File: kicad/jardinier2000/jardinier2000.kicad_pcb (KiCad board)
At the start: 2 copper layers, 54 parts, among them J1 5V, J10 I2C, J11 I2C, J12 Barrel_Jack_Switch, J2 VIN Reg, J3 5V, J4 5V, J5 5V, J6 5_30V, J7 I2C, J8 5V, J9 I2C, Q1 AO3400A, Q2 AO3400A, Q3 AO3400A, Q4 AO3400A, Q5 AO3400A, Q6 AO3400A, U1 ESP32_DevKit_V1_DOIT, U2 NCP1117-3.3_SOT223, U3 TPS62933P

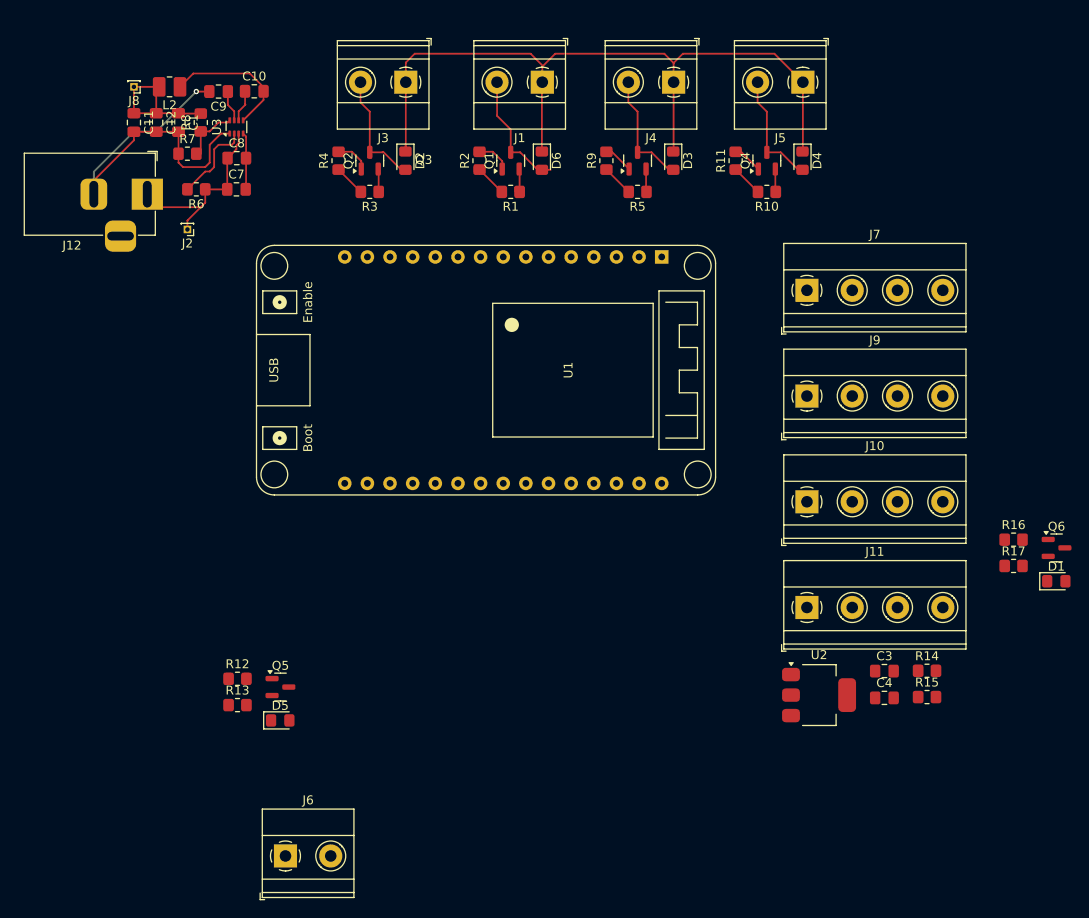
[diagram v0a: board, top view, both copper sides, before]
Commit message: Finished routing v1.0
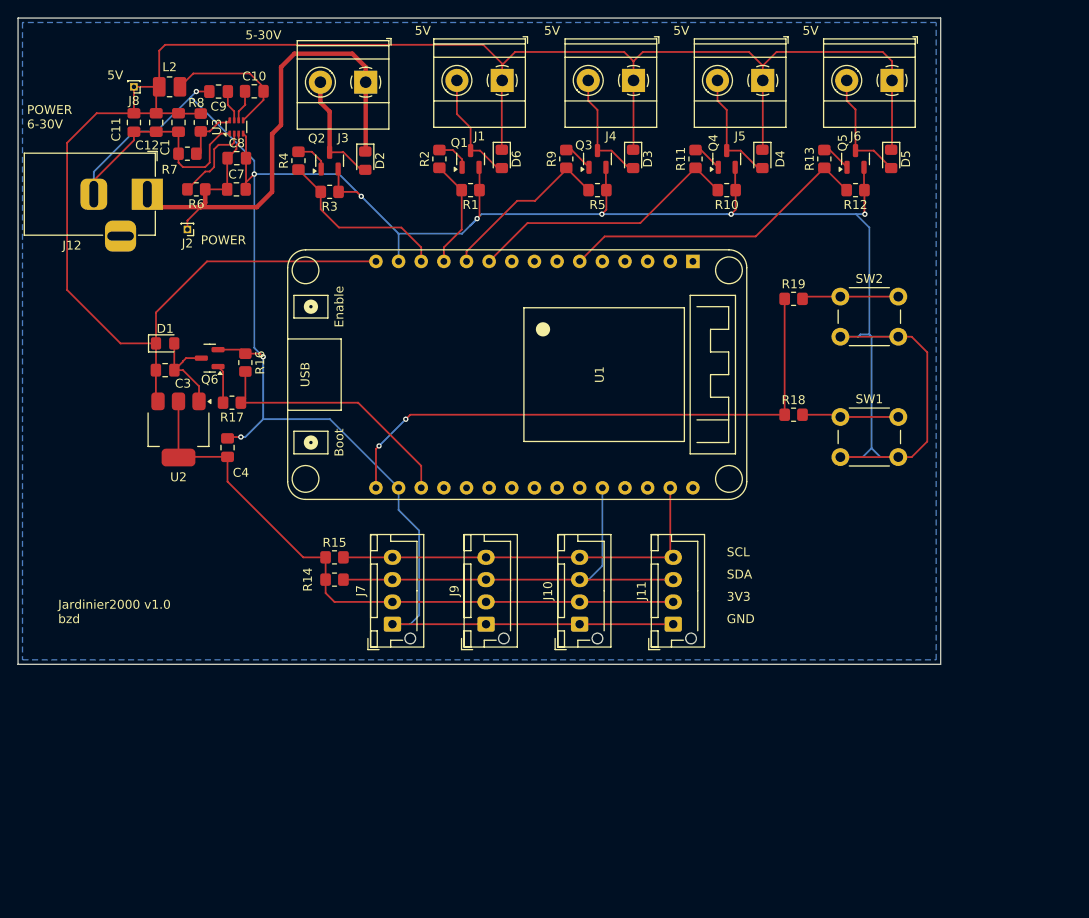
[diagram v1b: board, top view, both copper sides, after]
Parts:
- added R18: 10K, Resistor_SMD:R_0805_2012Metric_Pad1.20x1.40mm_HandSolder, F.Cu at (154.0, 81.5)
- added R19: 10K, Resistor_SMD:R_0805_2012Metric_Pad1.20x1.40mm_HandSolder, F.Cu at (154.0, 68.5)
- added SW1: SW_Push, Button_Switch_THT:SW_PUSH_6mm, F.Cu at (159.2, 81.8)
- added SW2: SW_Push, Button_Switch_THT:SW_PUSH_6mm, F.Cu at (159.2, 68.2)
- J10, J11, J7, J9: footprint TerminalBlock_Phoenix:TerminalBlock_Phoenix_MKDS-1,5-4-5.08_1x04_P5.08mm_Horizontal -> Connector_JST:JST_XH_B4B-XH-AM_1x04_P2.50mm_Vertical
- J3: value 5V -> 5_30V
- J6: value 5_30V -> 5V
- moved J6 110.4 mm to (165.0, 44.0), turned to 180 degrees
- moved D1 103.5 mm to (83.5, 73.5)
- moved Q6 97.4 mm to (88.5, 75.2), turned to 180 degrees
- moved D5 93.1 mm to (164.9, 52.8), turned to -90 degrees
- moved R13 89.9 mm to (157.4, 52.8), turned to 90 degrees
- moved R17 89.6 mm to (91.0, 80.2), turned to 180 degrees
- moved R16 88.4 mm to (92.5, 75.7), turned to -90 degrees
- moved R12 88.4 mm to (160.9, 56.3), turned to 180 degrees
- moved Q5 87.6 mm to (160.9, 52.8), turned to 90 degrees
- moved C3 87.5 mm to (83.5, 76.5)
- moved C4 78.9 mm to (90.5, 85.2), turned to 90 degrees
- moved U2 77.8 mm to (85.0, 83.2), turned to -90 degrees
- moved R15 68.3 mm to (102.5, 97.5)
- moved R14 67.3 mm to (102.5, 100.0)
- moved J7 59.7 mm to (109.0, 105.0), turned to 90 degrees
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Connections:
- C3 pad 1: /MOSFET 3A5/V+ -> /5V
- D1 pad 1: /MOSFET 3A5/V+ -> /5V
- D2 pad 1: /5V -> /VDD_5_30V
- D5 pad 1: /VDD_5_30V -> /5V
- J3 pad 1: /5V -> /VDD_5_30V
- J6 pad 1: /VDD_5_30V -> /5V
- U1 pad 16: unconnected-(U1-3V3-Pad16) -> /ESP32_3V3
- U1 pad 18: unconnected-(U1-IO15-Pad18) -> /Trigger_3V3
- U1 pad 9: /Trigger_3V3 -> unconnected-(U1-IO26-Pad9)
- U2 pad 3: /MOSFET 3A5/V+ -> /5V
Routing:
- net GND: track 62.9 -> 349.3 mm, vias 1 -> 9
- net /5V: track 103.2 -> 221.5 mm
- net /3V3: track 0.00 -> 72.5 mm
- net /ESP32_3V3: track 0.00 -> 64.8 mm, vias 0 -> 2
- net /SDA: track 0.00 -> 48.9 mm
- net /SCL: track 0.00 -> 44.9 mm
- net /VDD_5_30V: track 21.2 -> 65.2 mm
- net /MOSFET 3A4/Trigger: track 0.00 -> 35.3 mm
- net /Trigger_3V3: track 0.00 -> 29.3 mm
- net /MOSFET 3A3/Trigger: track 3.54 -> 31.0 mm
- net /MOSFET 3A1/Trigger: track 3.54 -> 20.1 mm
- net /MOSFET 3A2/Trigger: track 3.54 -> 19.8 mm
- net /MOSFET 3A4/V-: track 0.00 -> 13.1 mm
- net /MOSFET 3A5/V-: track 0.00 -> 11.8 mm
- net Net-(R19-Pad2): track 0.00 -> 10.9 mm
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- added copper zone on B.Cu, net GND
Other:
- board outline added: 103.5 x 72.5 mm
- board text added: "3V3"
- board text added: "5-30V"
- board text added: "5V"
- board text added: "GND"
- board text added: "Jardinier2000 v1.0 bzd"
- board text added: "POWER"
- board text added: "POWER 6-30V"
- board text added: "SCL"
- board text added: "SDA"
